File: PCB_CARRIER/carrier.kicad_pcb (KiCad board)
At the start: 6 copper layers, 69.6 x 46 mm, 87 parts, among them J1 SODIMM-260_Split, J2 Micro_SD_Card_Det2, Q1 BSS138, Q2 BSS138, Q3 BSS138, Q4 BC817-40, SW1 SW_DIP_x04, U1 SN74LVC8T245, U2 SN74LVC8T245, U3 SN74LVC8T245, U4 RT9742GGJ5

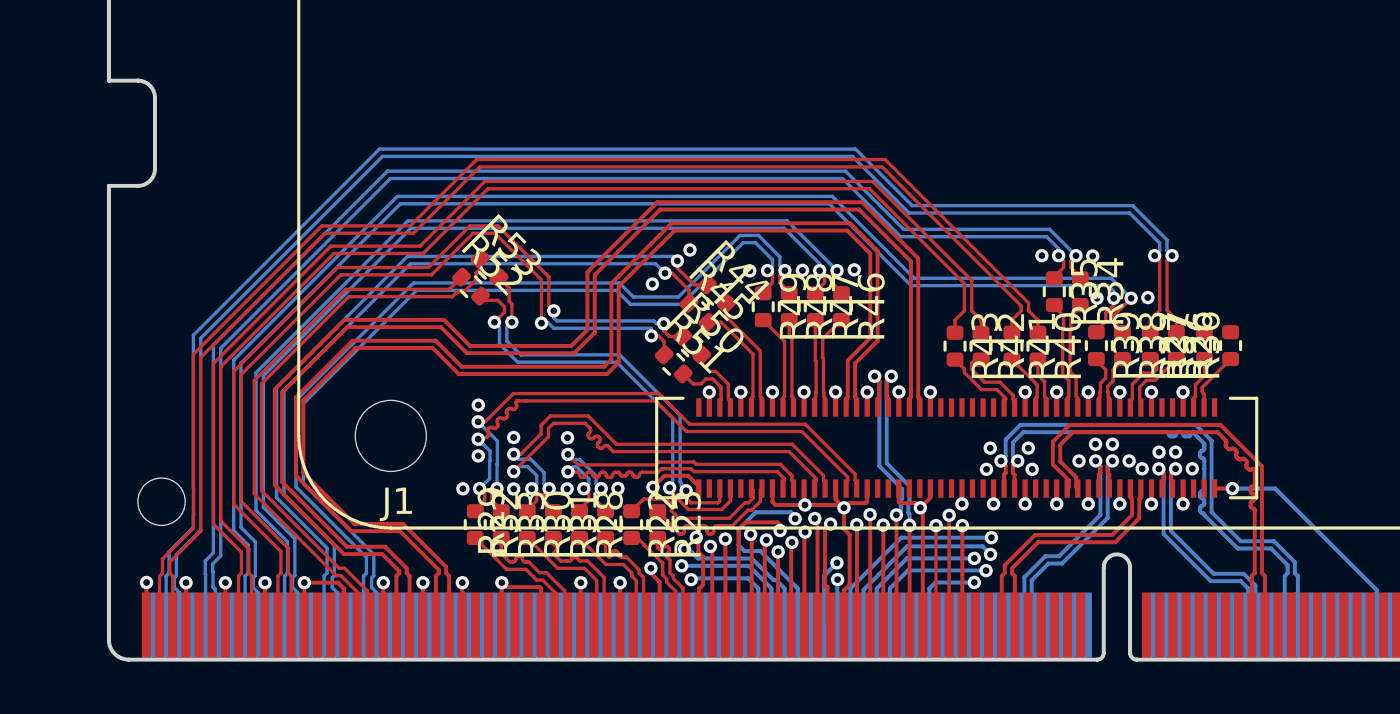
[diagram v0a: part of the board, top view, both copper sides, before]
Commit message: tuned skew before dampening resistors
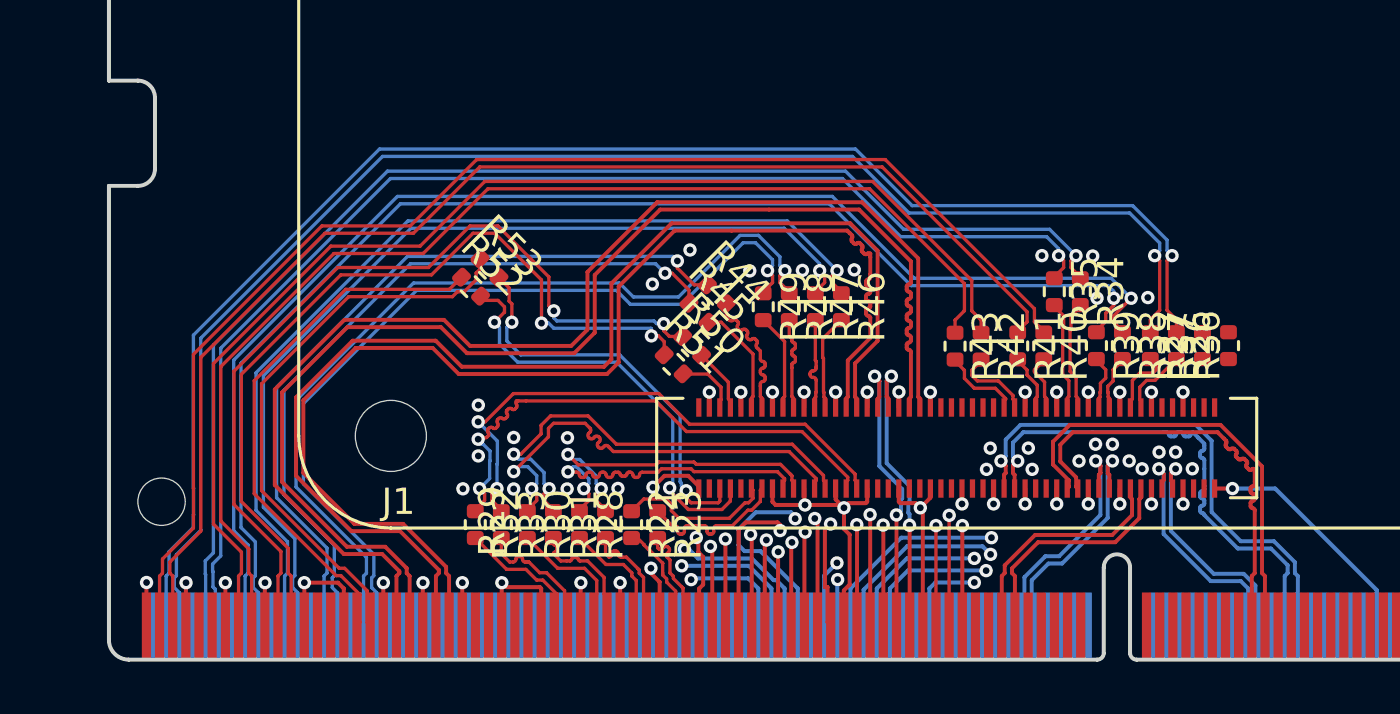
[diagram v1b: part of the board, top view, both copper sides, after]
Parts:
- moved R40 0.22 mm to (135.5, 88.1)
- moved R41 0.22 mm to (134.5, 88.1)
- moved R26 0.08 mm to (142.5, 88.1)
- moved R27 0.08 mm to (141.6, 88.1)
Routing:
- net USB_N: track 2.32 -> 0.00 mm
- net USB_P: track 2.01 -> 0.00 mm
- net CSI-1_CLK_N: track 4.50 -> 5.47 mm
- net USB3-1-RX_P: track 47.0 -> 47.8 mm
- net USB3-1-TX_P: track 45.2 -> 46.1 mm

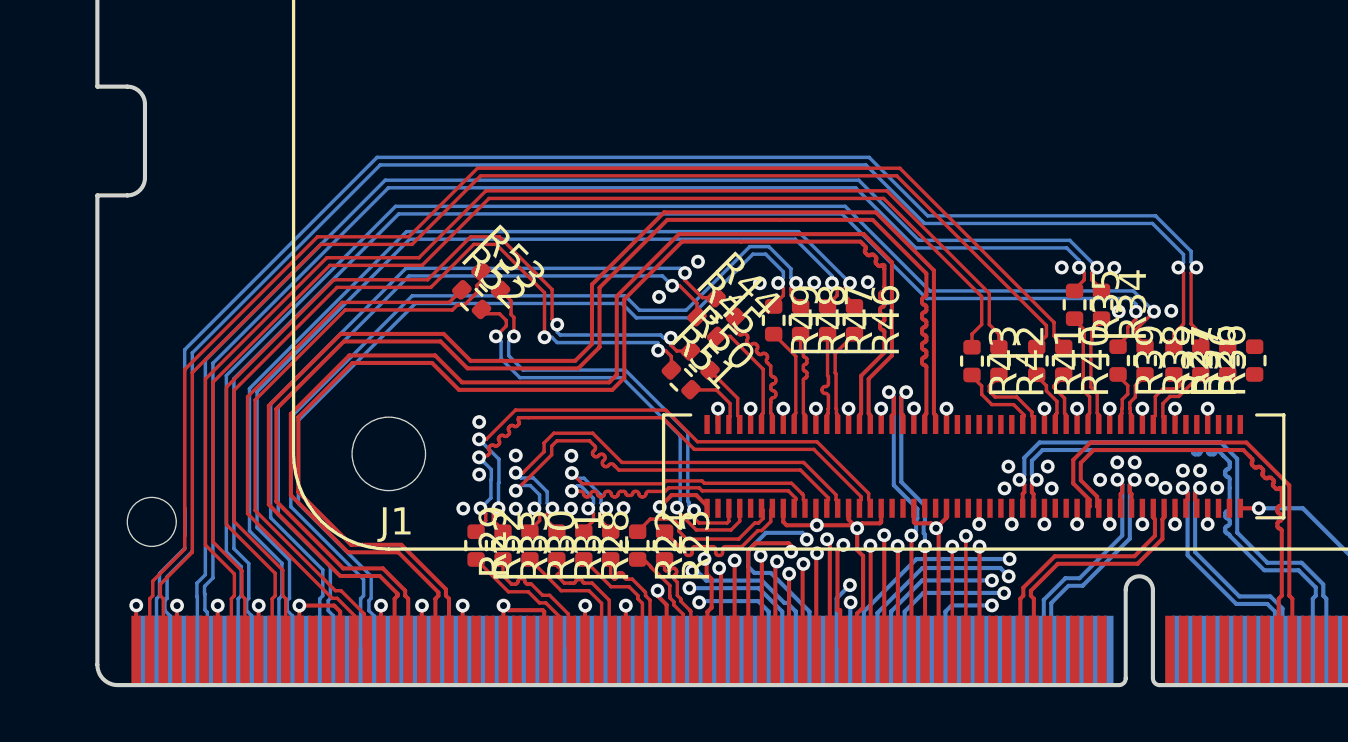
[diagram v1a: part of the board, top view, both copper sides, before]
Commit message: tuned the skew of every CSI line, done CSI and some DP/DMgit add .!
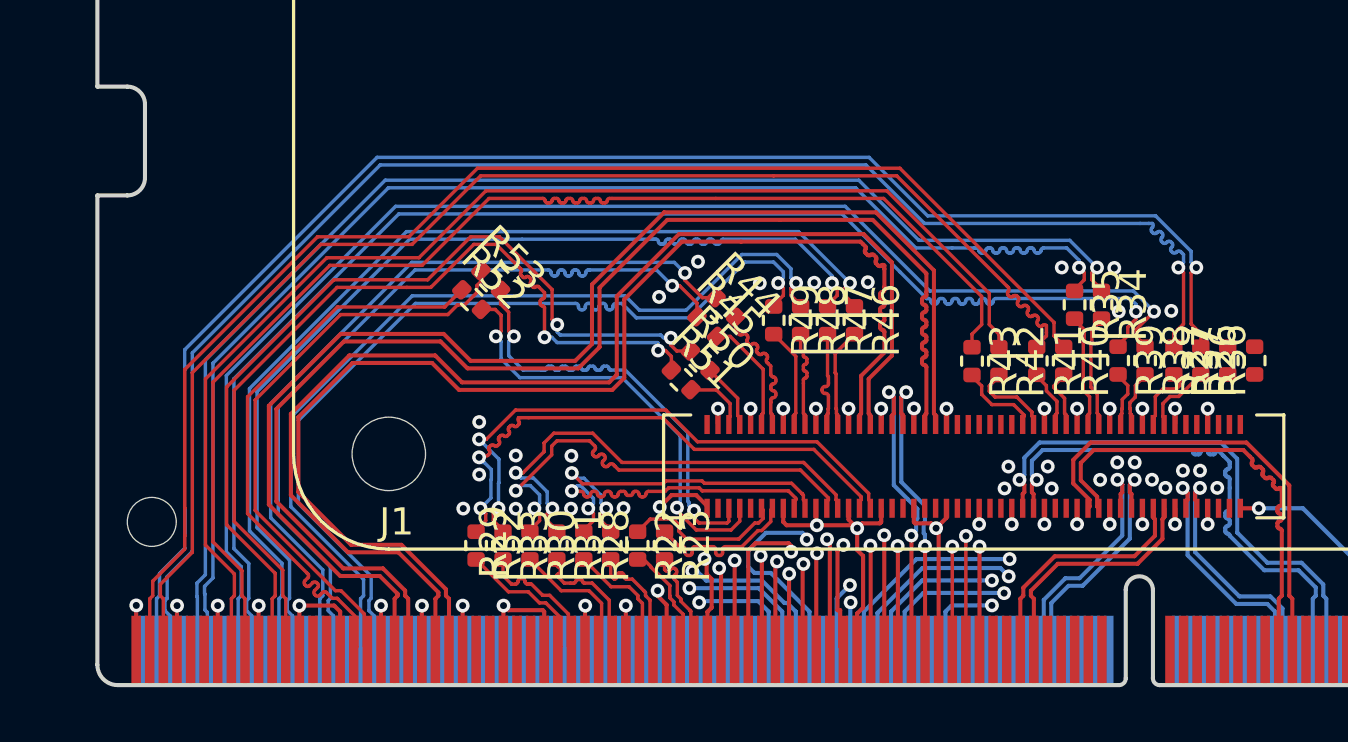
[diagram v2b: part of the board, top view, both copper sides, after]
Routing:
- net dCSI-0_D1_P: track 49.2 -> 50.3 mm
- net dCSI-1_D3_N: track 20.6 -> 21.7 mm
- net dCSI-0_CLK_P: track 47.7 -> 48.7 mm
- net dCSI-1_D0_P: track 35.5 -> 36.4 mm
- net dCSI-1_CLK_P: track 28.1 -> 29.1 mm
- net dCSI-0_D2_P: track 48.3 -> 49.2 mm
- net dCSI-0_D3_P: track 44.9 -> 45.7 mm
- net dCSI-0_D0_P: track 55.8 -> 56.6 mm
- net CSI-1_D3_P: track 15.5 -> 16.3 mm
- net dCSI-1_D1_P: track 32.3 -> 32.9 mm
